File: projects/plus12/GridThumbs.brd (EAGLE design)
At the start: 116.2 x 25.4 mm, 15 parts

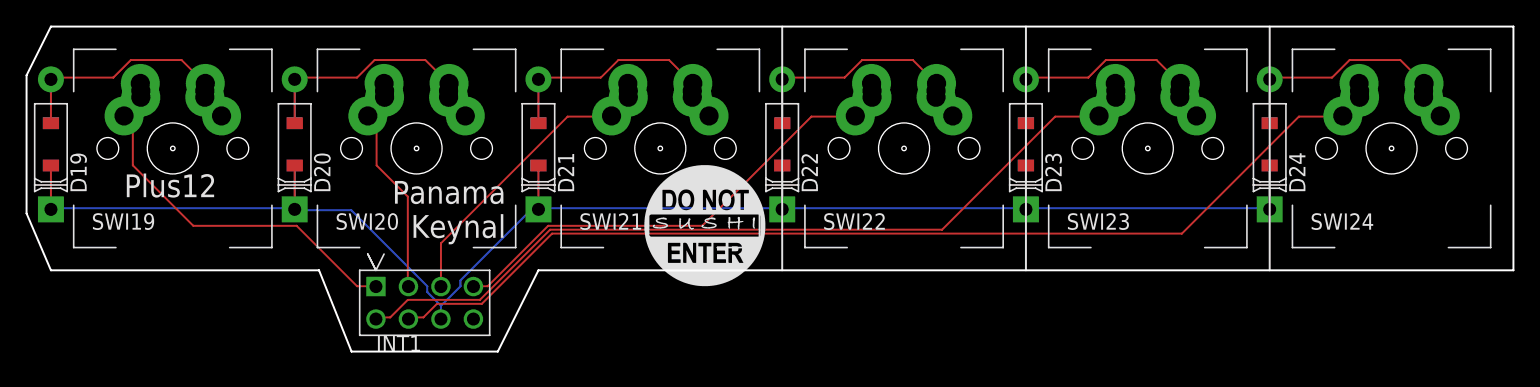
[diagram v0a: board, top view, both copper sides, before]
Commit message: more updates than should be in one commit, lots of work
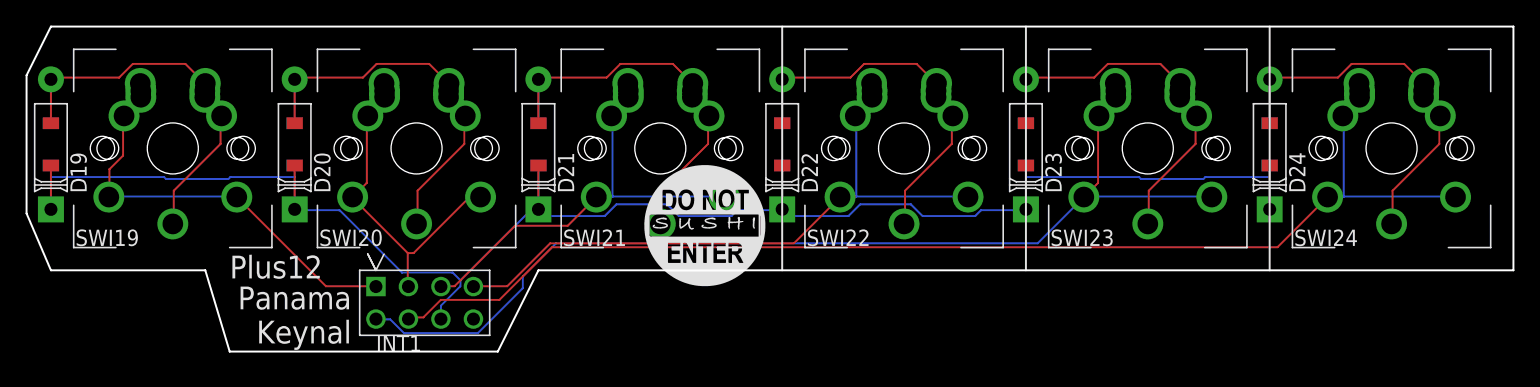
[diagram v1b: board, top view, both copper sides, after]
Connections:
- net N$10: now also SWI22.RLMID
- net N$11: now also SWI23.RLMID
- net N$12: now also SWI24.RLMID
- net N$2: now also SWI20.LLP, SWI20.LRLP
- net N$21: now also SWI19.LLP, SWI19.LRLP
- net N$3: now also SWI21.LLP, SWI21.LRLP
- net N$4: now also SWI22.LLP, SWI22.LRLP
- net N$5: now also SWI23.LLP, SWI23.LRLP
- net N$6: now also SWI24.LLP, SWI24.LRLP
- net N$7: now also SWI19.RLMID
- net N$8: now also SWI20.RLMID
- net N$9: now also SWI21.RLMID
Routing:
- net N$7: track 20.9 -> 34.9 mm
- net N$9: track 20.9 -> 34.9 mm
- net N$11: track 20.9 -> 34.9 mm
- net N$12: track 21.4 -> 34.9 mm
- net N$8: track 21.4 -> 34.9 mm
- net N$10: track 21.4 -> 34.9 mm
- net N$5: track 68.5 -> 80.9 mm
- net N$6: track 84.9 -> 96.3 mm
- net N$4: track 40.7 -> 52.0 mm
- net N$3: track 26.2 -> 35.5 mm
- net N$2: track 20.0 -> 27.3 mm
- net N$19: track 144.3 -> 147.5 mm
- net N$21: track 32.4 -> 34.5 mm
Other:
- outline, holes or cut-outs redrawn
